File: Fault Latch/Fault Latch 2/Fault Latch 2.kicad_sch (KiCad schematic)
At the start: 114 parts, among them J1 1053141312, J3 1053131202, J4 1053131202, K101 Fujitsu_FTR-LYAA005x, K102 Fujitsu_FTR-LYAA005x, K103 Fujitsu_FTR-LYAA005x, Q101 Q_NPN_BEC, Q102 Q_NPN_BEC, Q103 Q_NPN_BEC, Q104 Q_NPN_BEC, Q105 Q_NMOS_GSD, Q106 Q_NMOS_GSD, Q107 Q_PMOS_GSD, Q108 Q_PMOS_GSD, Q109 Q_PMOS_GSD, Q110 Q_NPN_BEC, Q111 Q_NPN_BEC, Q112 Q_NMOS_GSD, Q113 Q_NMOS_GSD, Q114 Q_NMOS_GSD, Q115 Q_NMOS_GSD, Q116 Q_NMOS_GSD, SW101 SW_Omron_B3FS, SW102 SW_Omron_B3FS, SW103 SW_Omron_B3FS, U101 SFH617A-1, U102 SFH617A-1, U103 SFH617A-1, U104 74AHC1G00, U105 74AHC1G00, U106 74AHC1G00, U107 74LS279, U109 SFH617A-1, U110 SFH617A-1, U117 74AHC1G00, U118 LM555xM, U119 74AHC1G00, U121 SFH617A-1, U2 LM1117DT-5.0

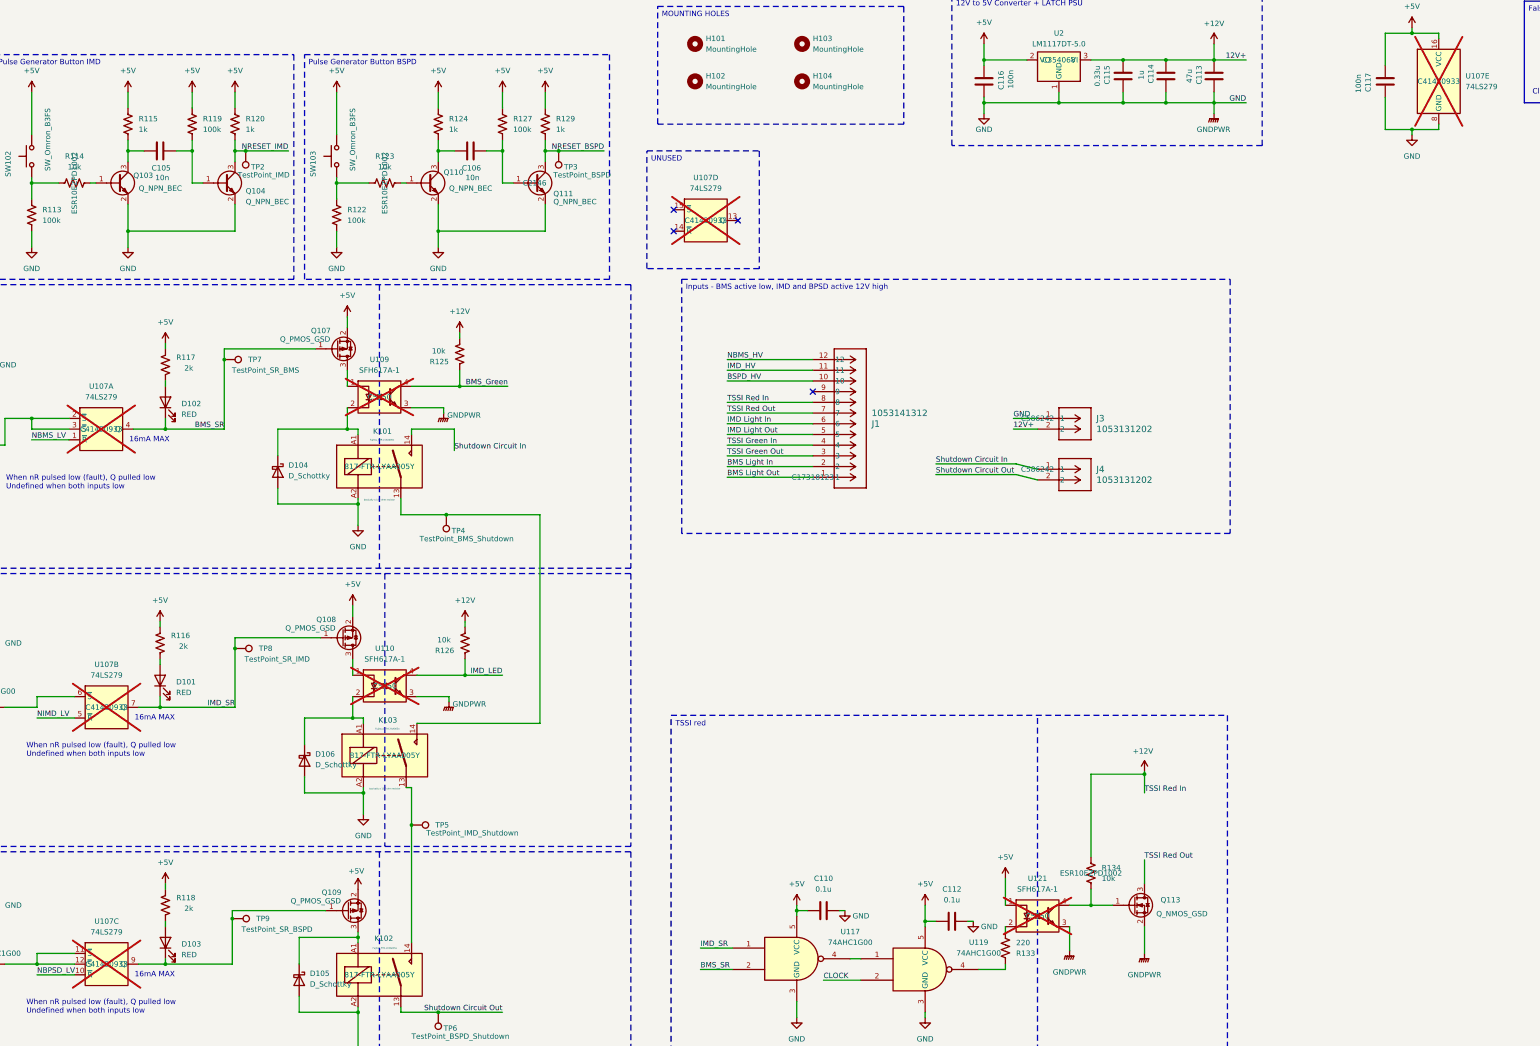
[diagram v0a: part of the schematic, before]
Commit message: BOM stuff
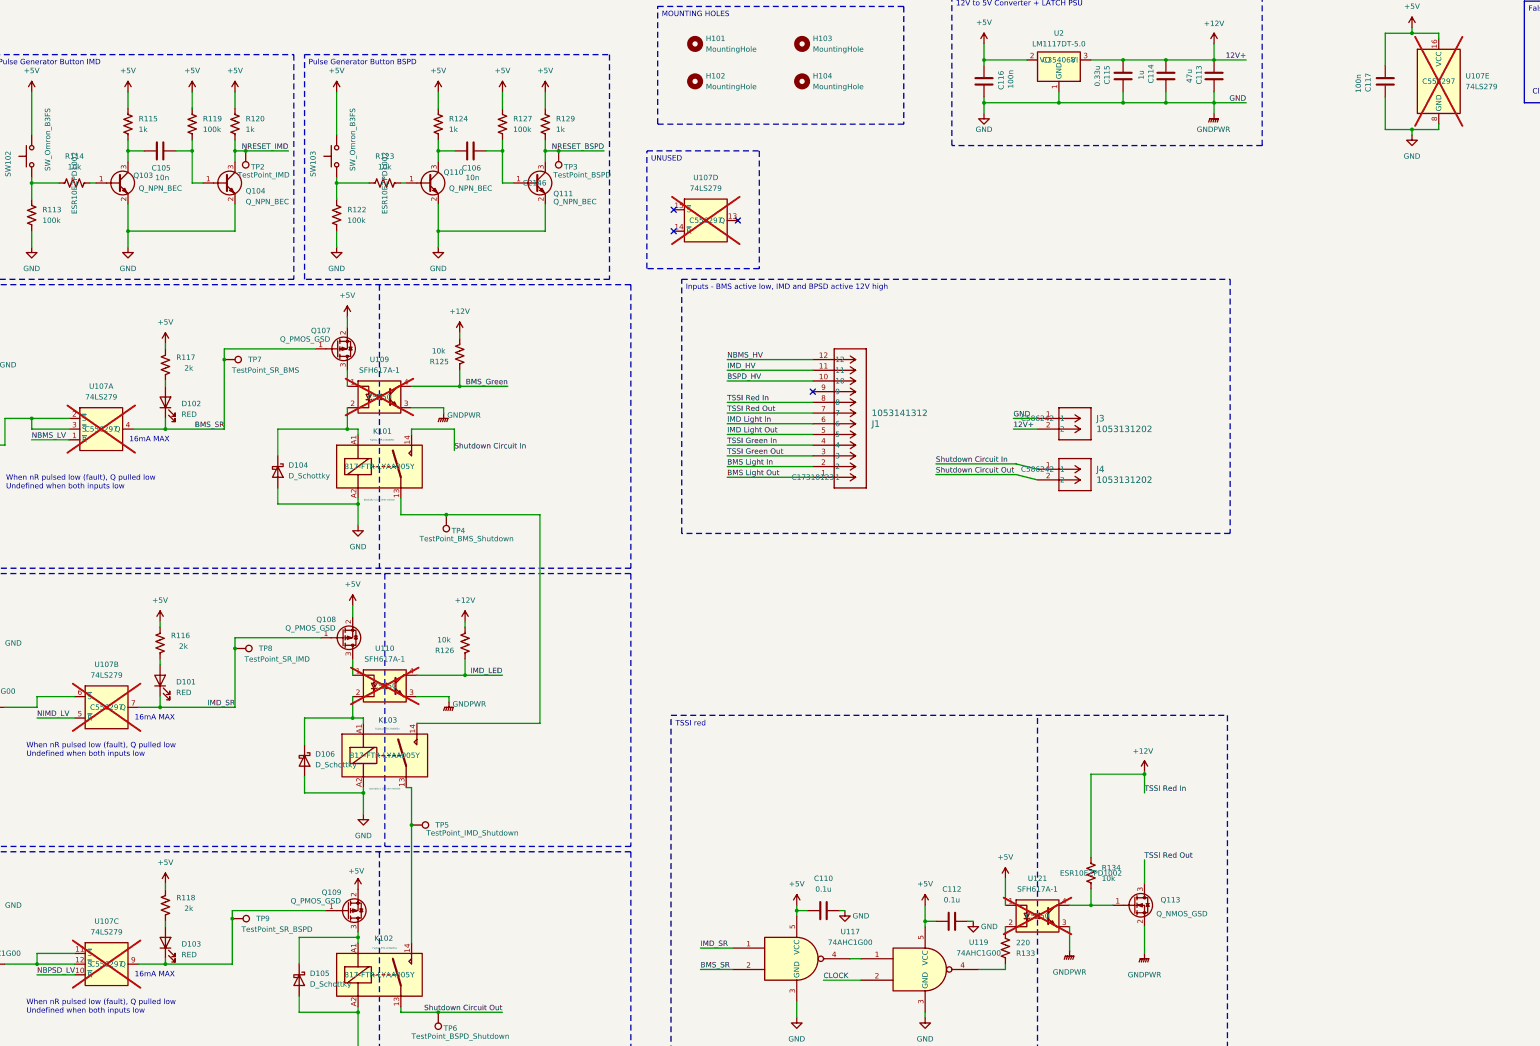
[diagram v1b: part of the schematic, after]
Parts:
- R102, R103, R104, R133: JLC# C2074007 -> C17557
- R116, R117, R118: JLC# C2889470 -> C1359
- U107: JLC# C41430933 -> C556297
- U118: JLC# C90760 -> (none)
